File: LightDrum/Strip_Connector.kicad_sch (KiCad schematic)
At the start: 29 parts, among them J3 0366380003

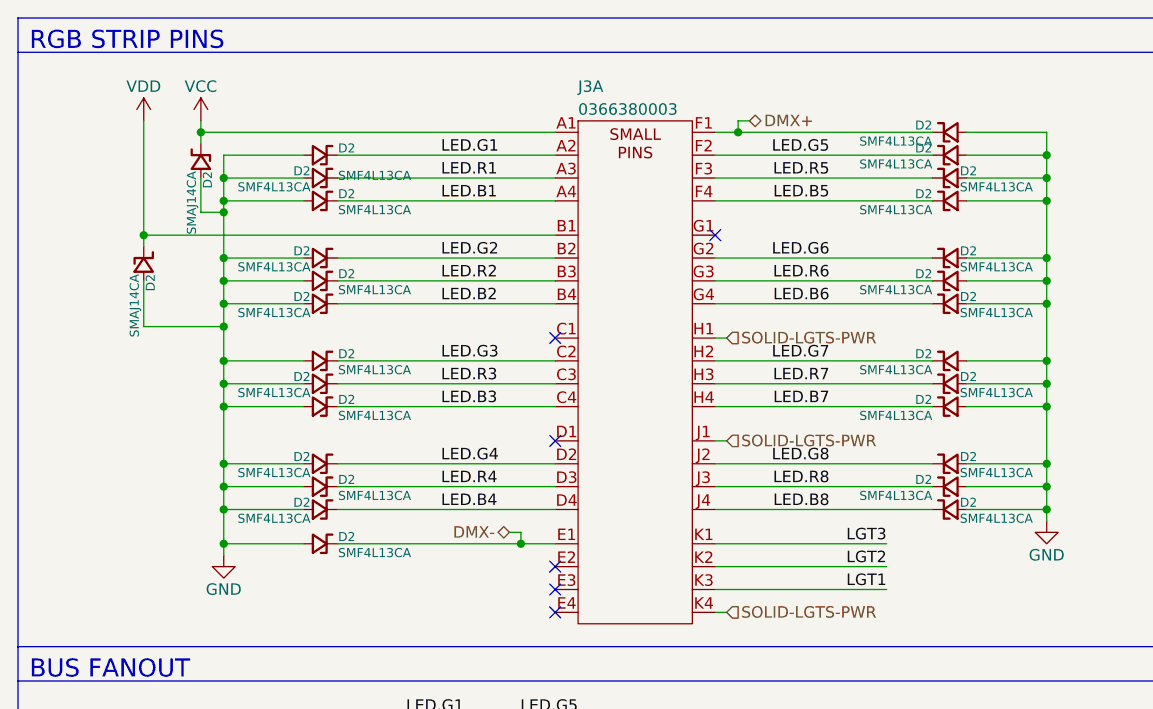
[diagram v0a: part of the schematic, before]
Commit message: REV13 - Update to KiCAD 8
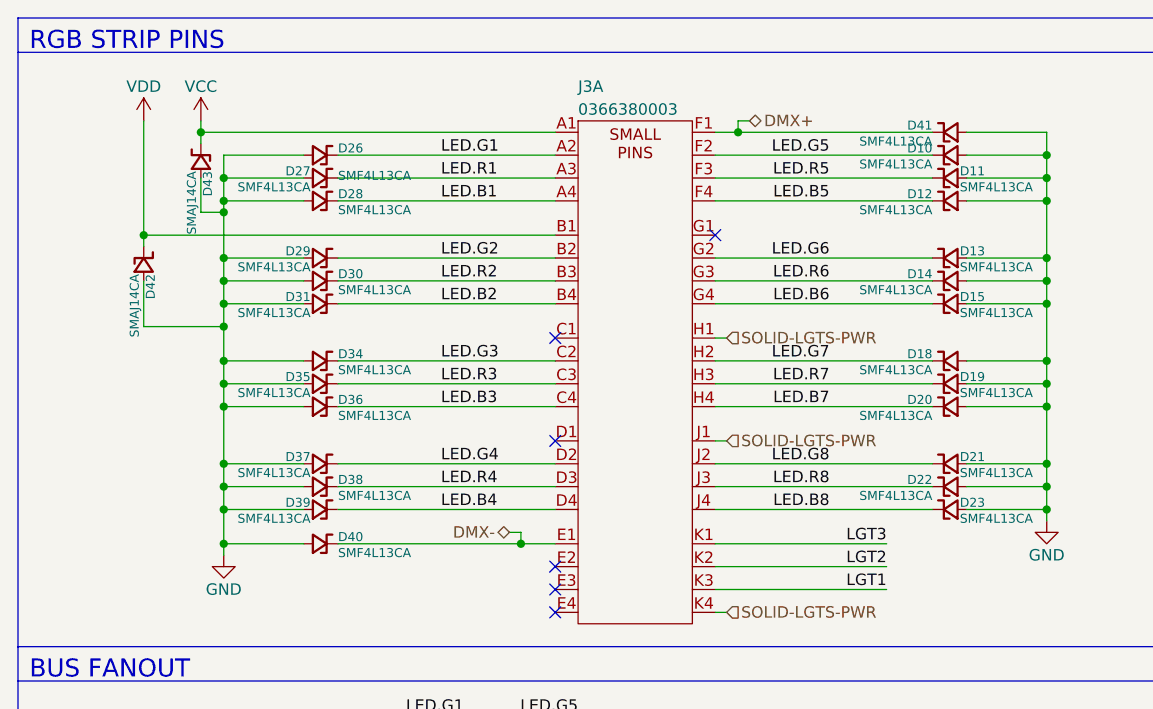
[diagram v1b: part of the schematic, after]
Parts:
- renumbered D2 to D10, D2 to D11, D2 to D12, D2 to D13, D2 to D14, D2 to D15, D2 to D18, D2 to D19, D2 to D20, D2 to D21, D2 to D22, D2 to D23, D2 to D26, D2 to D27, D2 to D28, D2 to D29, D2 to D30, D2 to D31, D2 to D34, D2 to D35, D2 to D36, D2 to D37, D2 to D38, D2 to D39, D2 to D40, D2 to D41, D2 to D42, D2 to D43

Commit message: REV13 - Revert to KiCAD 7
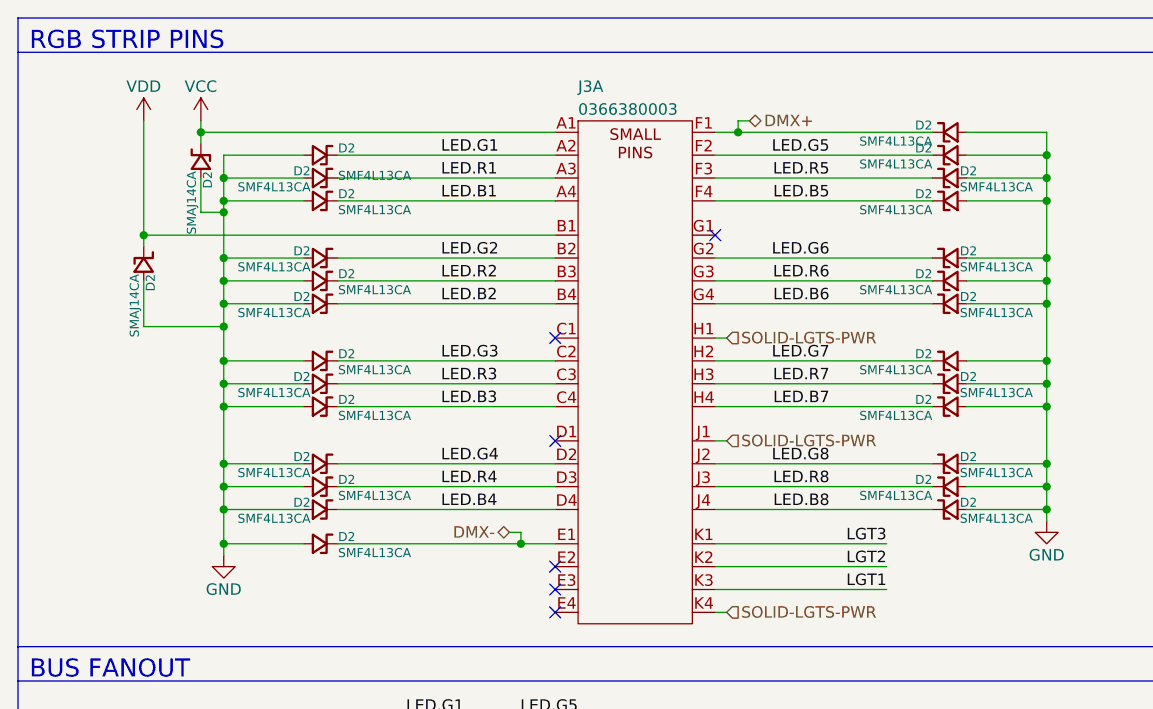
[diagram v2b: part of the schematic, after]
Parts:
- renumbered D30 to D2, D14 to D2, D23 to D2, D18 to D2, D22 to D2, D19 to D2, D10 to D2, D37 to D2, D38 to D2, D26 to D2, D40 to D2, D42 to D2, D29 to D2, D27 to D2, D20 to D2, D15 to D2, D34 to D2, D35 to D2, D28 to D2, D39 to D2, D43 to D2, D36 to D2, D13 to D2, D12 to D2, D41 to D2, D31 to D2, D11 to D2, D21 to D2
